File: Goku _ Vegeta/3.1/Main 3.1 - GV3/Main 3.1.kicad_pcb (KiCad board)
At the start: 2 copper layers, 206 x 197.4 mm, 74 parts, among them J1 Battery Buzzer, J10 Motor 4, J11 LEFT HEADERS, J12 RIGHT HEADERS, J13 MID HEADERS, J14 UART, J15 I2C, J16 4S Battery, J17 Power Switch, J18 Batt Bal, J19 5V PI, J20 ESC PWR, J21 Line, J23 ESC PWM, J3 BACKUP 3V3, J5 SPI, J6 Solenoid, J7 Motor 1, J8 Motor 2, J9 Motor 3, Q1 BSC040N10NS5, Q2 Q_Photo_NPN, U13 Adafruit_BNO055_STEMMA_QT, U15 Bluetooth_Module_(HC-05), U16 Bluetooth_Module_(HC-06), U4 TB67H420FTG Dual/Single Motor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, U5 TB67H420FTG Dual/Single Motor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, U6 TB67H420FTG Dual/Single Motor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, U7 TB67H420FTG Dual/Single Motor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, U8 DEV-16771, U9 Arduino Compatible DC-DC Boos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

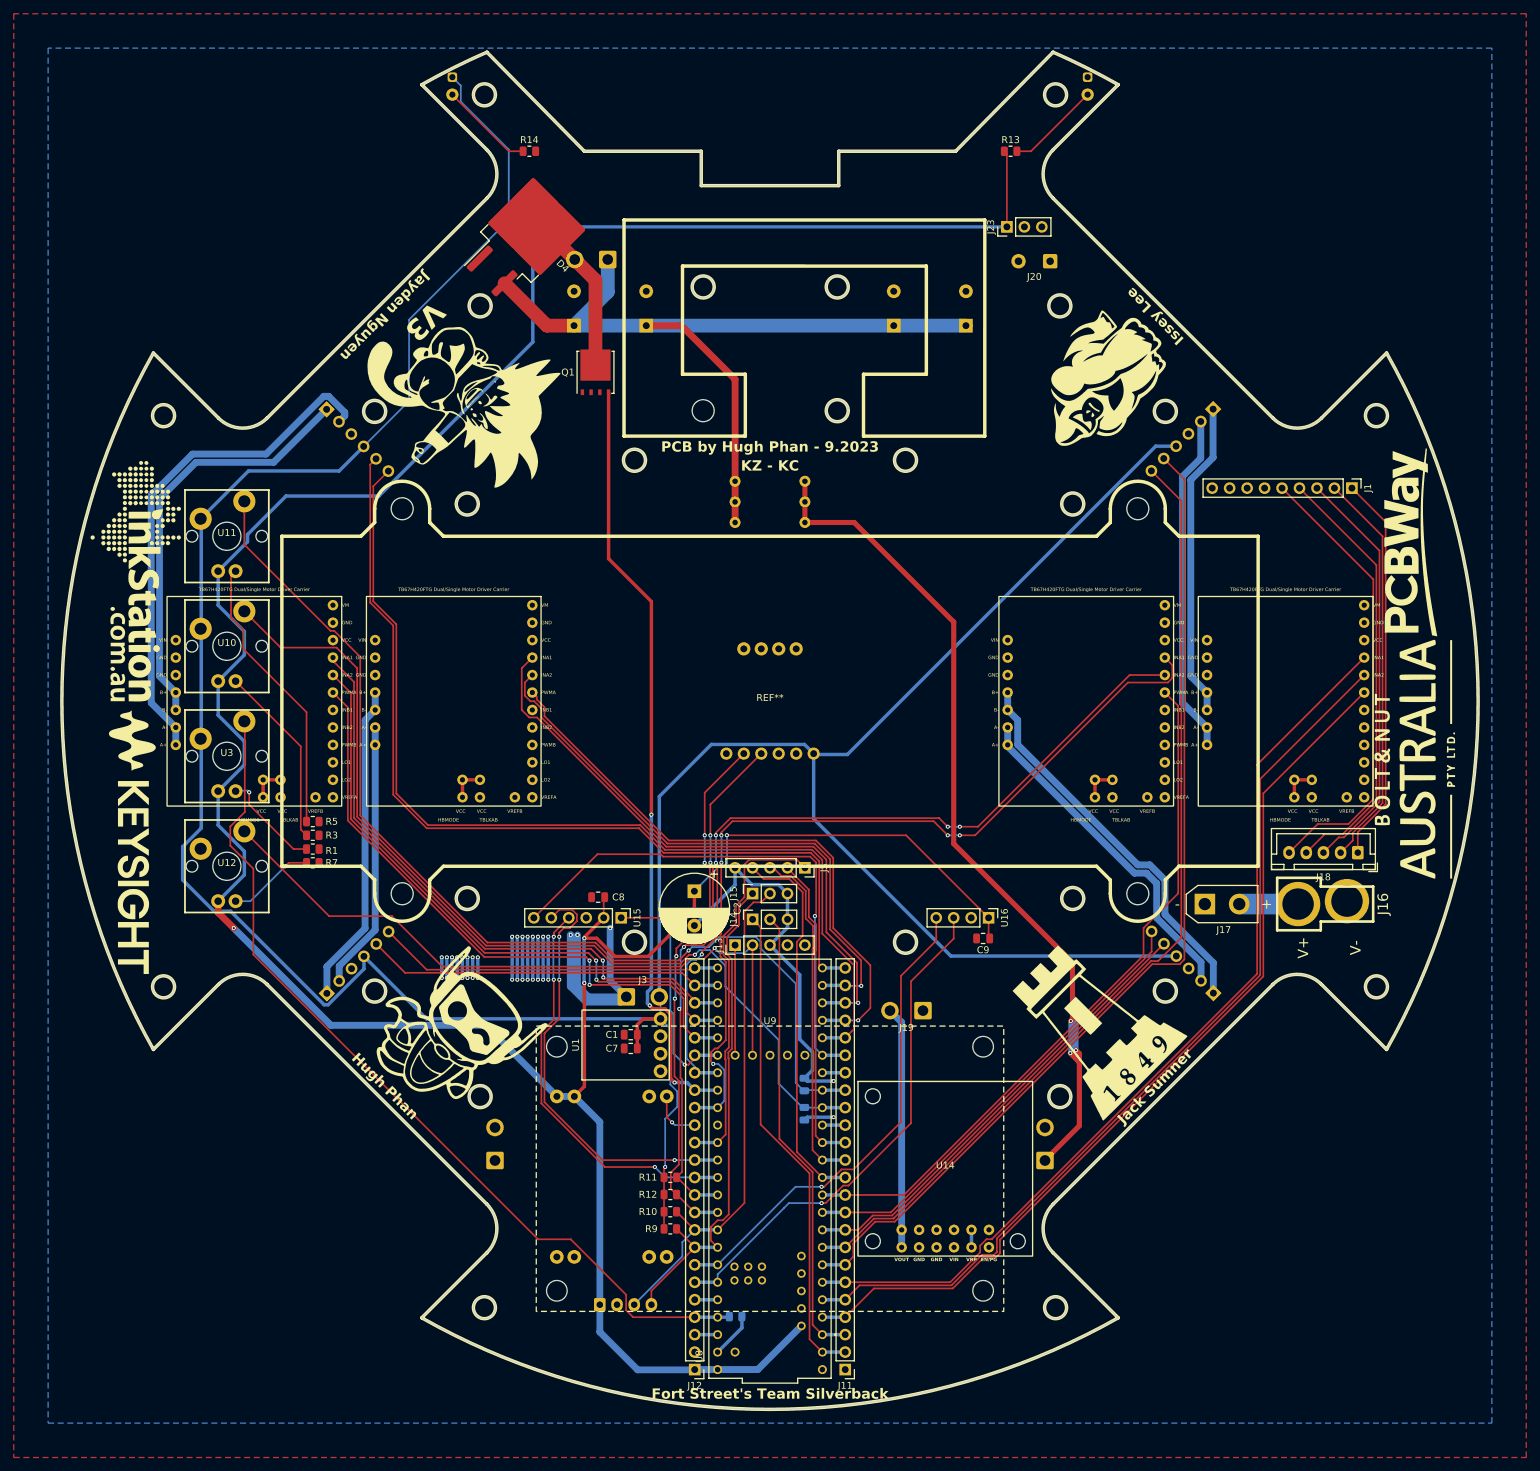
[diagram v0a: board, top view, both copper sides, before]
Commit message: main 3.1 edit actualy done now i think...
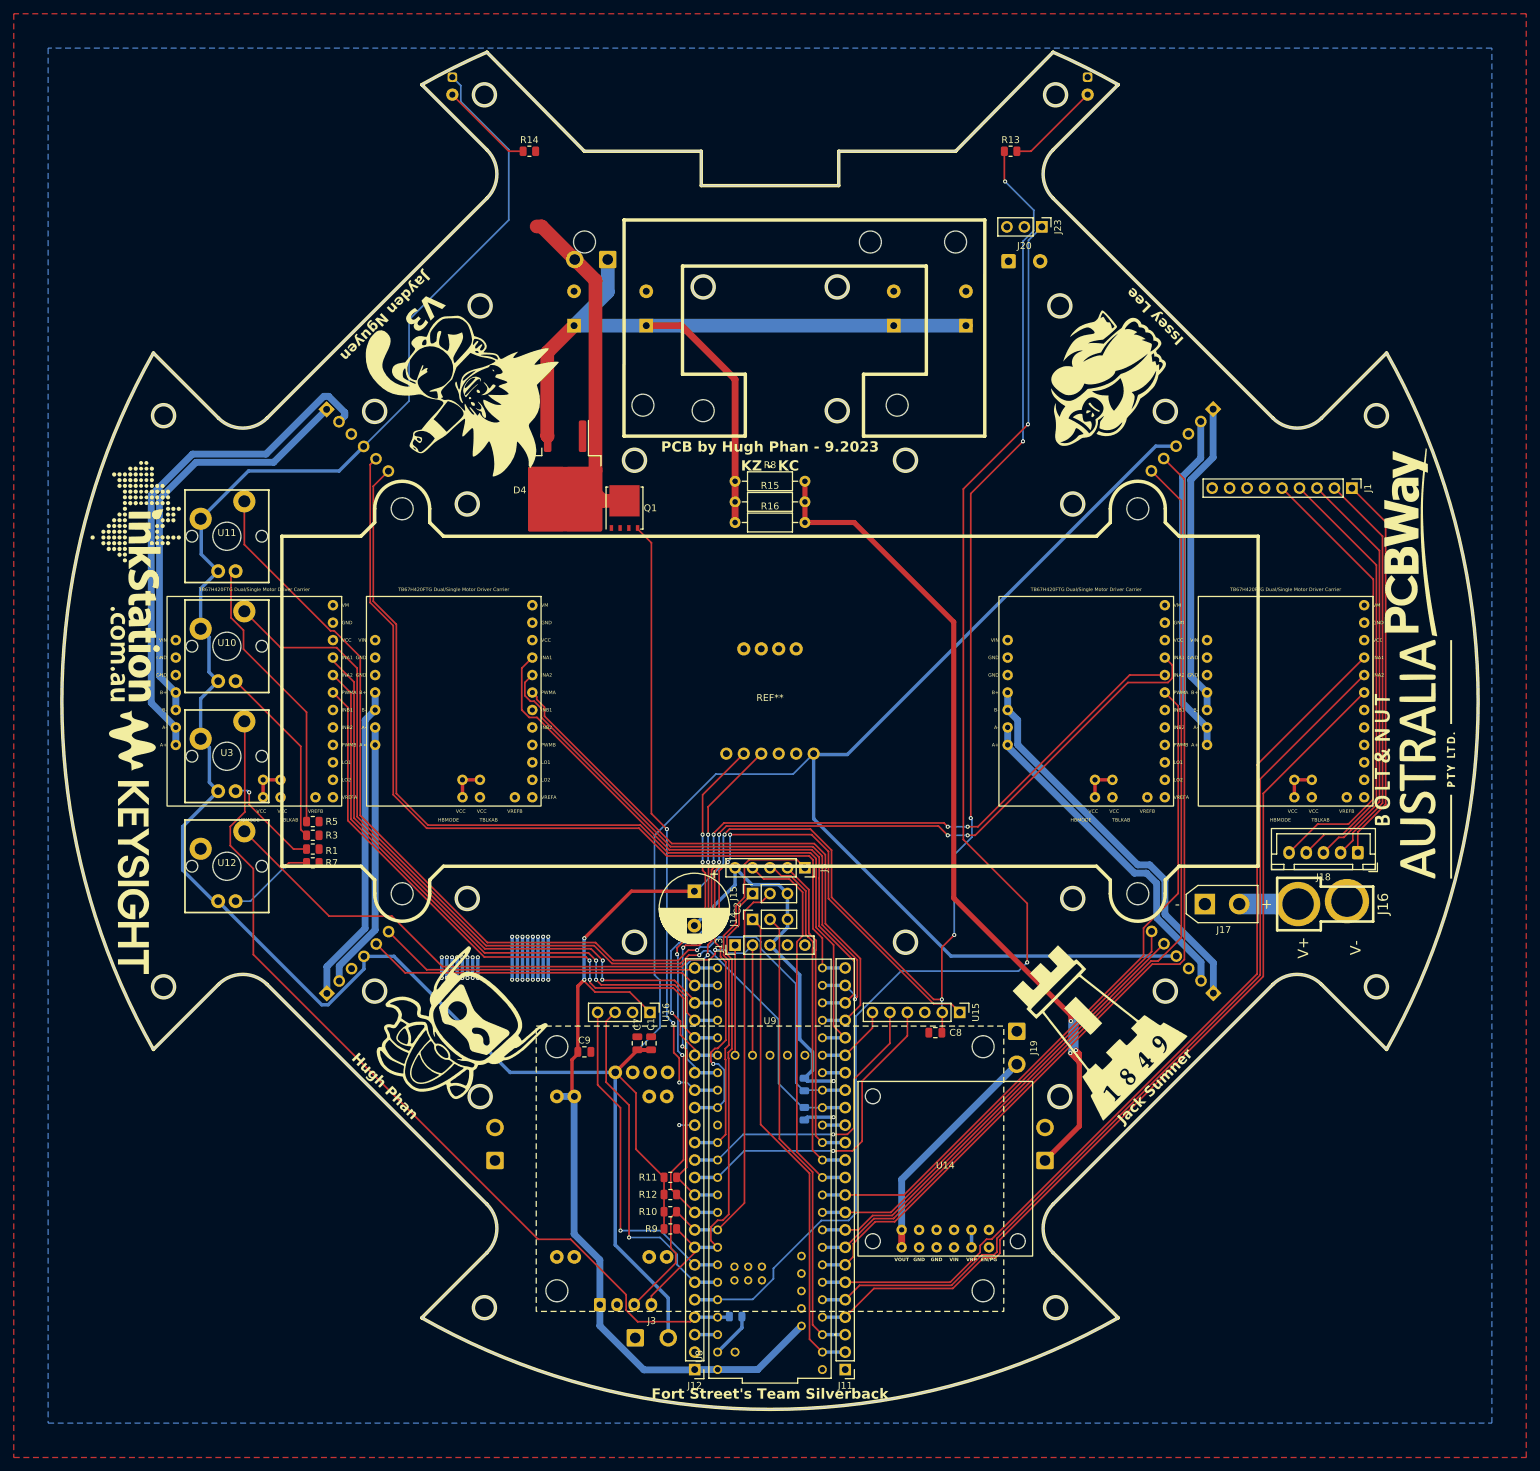
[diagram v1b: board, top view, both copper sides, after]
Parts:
- R15, R16, R8: moved to F.Cu
- U1: moved to B.Cu
- moved C9 60.3 mm to (123.0, 201.0), turned to 0 degrees
- moved C8 52.9 mm to (174.1, 198.2)
- moved U15 51.1 mm to (177.6, 195.2)
- moved U16 51.1 mm to (132.6, 195.2)
- moved J3 49.6 mm to (130.4, 242.6)
- moved D4 37.5 mm to (120.2, 119.1), turned to -90 degrees
- moved Q1 20.2 mm to (128.8, 121.9)
- moved J19 14.0 mm to (185.9, 198.0), turned to -90 degrees
- moved J20 6.05 mm to (184.7, 86.0), turned to 0 degrees
- moved R16 6.00 mm to (144.9, 124.0)
- moved R8 6.00 mm to (144.9, 118.0)
- moved J23 5.08 mm to (189.5, 81.0), turned to -90 degrees
- moved C1 3.20 mm to (132.7, 199.8), turned to 90 degrees
- moved U1 2.55 mm to (131.3, 198.9), turned to 180 degrees
- moved G*** 1.65 mm to (106.2, 104.4)
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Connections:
- J23 pad 1: +5V -> /22
- U10 pad A: +5V -> +3V3
- U11 pad A: +5V -> +3V3
- U12 pad A: +5V -> +3V3
- U3 pad A: +5V -> +3V3
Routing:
- net /22: track 3.33 -> 201.9 mm, vias 0 -> 2
- net +5V: track 455.8 -> 318.4 mm, vias 4 -> 8
- net /27: track 77.3 -> 11.2 mm, vias 1 -> 0
- net /38: track 34.6 -> 90.7 mm, vias 2 -> 4
- net GND: track 191.0 -> 142.7 mm, vias 38 -> 35
- net +3V3: track 472.5 -> 518.0 mm, vias 1 -> 0
- net Net-(D4-K): track 24.1 -> 48.9 mm
- net /40: track 112.6 -> 89.2 mm
- net /21: track 74.2 -> 51.1 mm
- net /20: track 70.4 -> 49.3 mm
- net /14: track 62.9 -> 44.1 mm, vias 3 -> 1
- net /15: track 58.8 -> 48.0 mm, vias 3 -> 1
- net Net-(D4-A): track 118.3 -> 123.4 mm
- net /29: track 86.5 -> 83.8 mm, vias 1 -> 0
- net /18: track 74.3 -> 76.4 mm
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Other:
- outline, holes or cut-outs redrawn
